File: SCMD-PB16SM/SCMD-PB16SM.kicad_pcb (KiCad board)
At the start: 2 copper layers, 200 x 100 mm, 26 parts, among them M1 SCMD, M10 SCMD, M11 SCMD, M12 SCMD, M2 SCMD, M3 SCMD, M4 SCMD, M5 SCMD, M6 SCMD, M7 SCMD, M8 SCMD, M9 SCMD

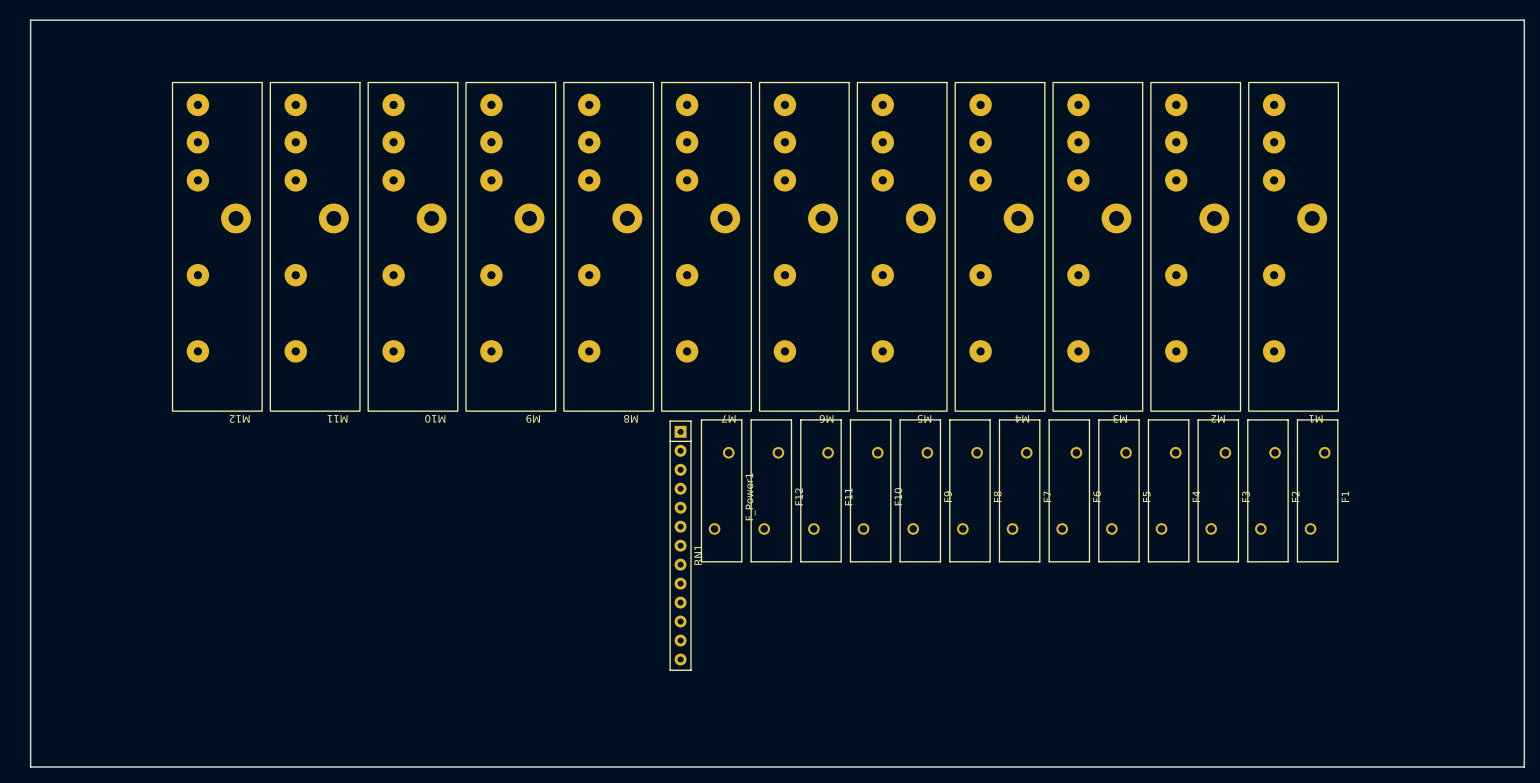
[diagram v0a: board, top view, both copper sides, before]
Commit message: Add files via upload
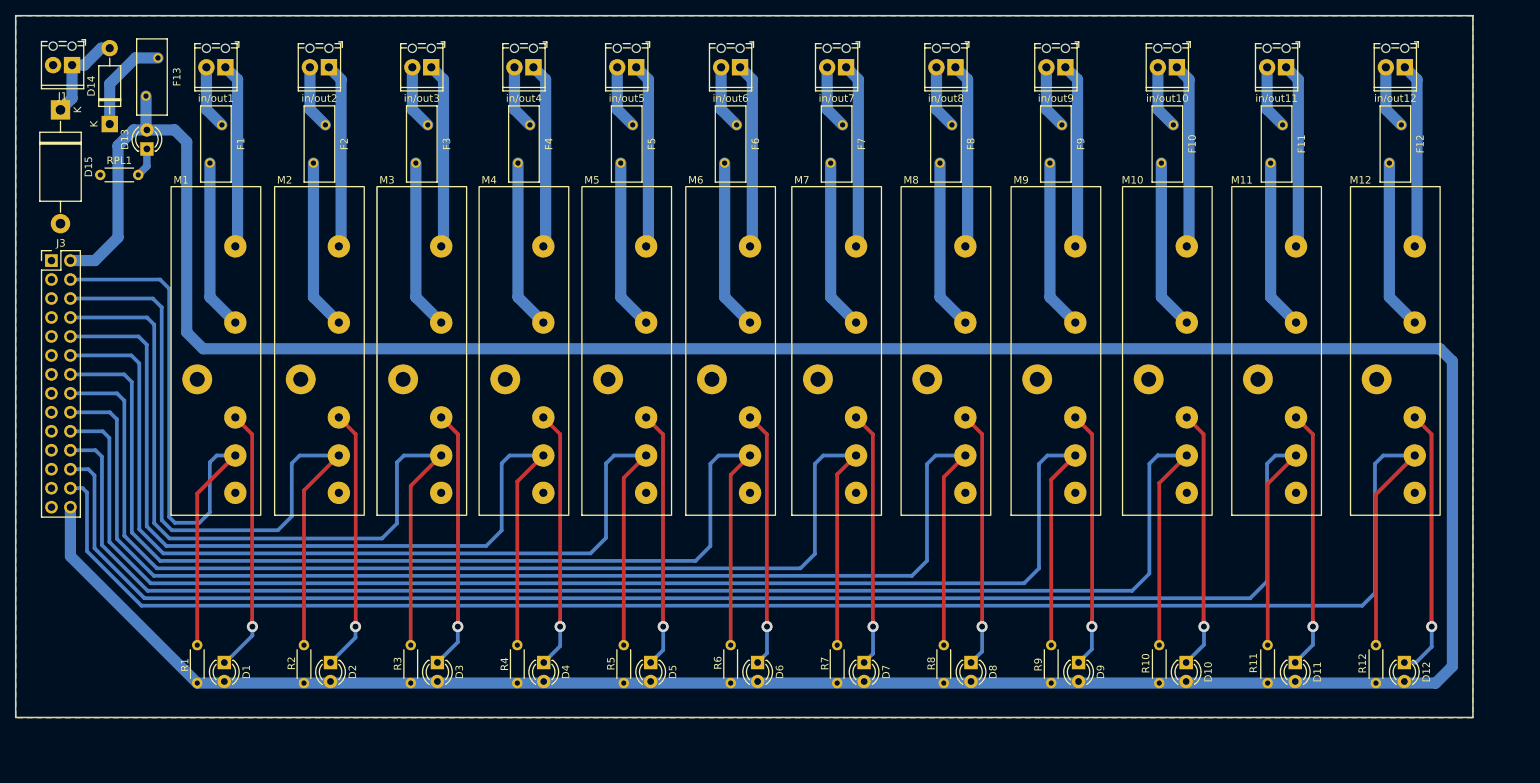
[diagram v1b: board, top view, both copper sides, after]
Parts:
- removed RN1: R_Network12, Resistor_THT:R_Array_SIP13
- added D1: LED, LED_THT:LED_D3.0mm_Clear, F.Cu at (53.9, 103.6)
- added D10: LED, LED_THT:LED_D3.0mm_Clear, F.Cu at (182.7, 103.6)
- added D11: LED, LED_THT:LED_D3.0mm_Clear, F.Cu at (197.3, 103.6)
- added D12: LED, LED_THT:LED_D3.0mm_Clear, F.Cu at (211.9, 103.6)
- added D13: LED, LED_THT:LED_D3.0mm_Clear, F.Cu at (43.6, 34.8)
- added D14: 1N4001, Diode_THT:D_DO-41_SOD81_P10.16mm_Horizontal, F.Cu at (38.6, 31.5)
- added D15: 1N62xxA, Diode_THT:D_DO-201AE_P15.24mm_Horizontal, F.Cu at (32.0, 29.6)
- added D2: LED, LED_THT:LED_D3.0mm_Clear, F.Cu at (68.2, 103.6)
- added D3: LED, LED_THT:LED_D3.0mm_Clear, F.Cu at (82.5, 103.6)
- added D4: LED, LED_THT:LED_D3.0mm_Clear, F.Cu at (96.7, 103.6)
- added D5: LED, LED_THT:LED_D3.0mm_Clear, F.Cu at (111.0, 103.6)
- added D6: LED, LED_THT:LED_D3.0mm_Clear, F.Cu at (125.3, 103.6)
- added D7: LED, LED_THT:LED_D3.0mm_Clear, F.Cu at (139.6, 103.6)
- added D8: LED, LED_THT:LED_D3.0mm_Clear, F.Cu at (153.9, 103.6)
- added D9: LED, LED_THT:LED_D3.0mm_Clear, F.Cu at (168.3, 103.6)
- added J1: Logic Supply, TerminalBlock_Phoenix:TerminalBlock_Phoenix_MPT-0,5-2-2.54_1x02_P2.54mm_Horizontal, F.Cu at (33.5, 23.6)
- added J3: Edge Connector, Connector_PinHeader_2.54mm:PinHeader_2x14_P2.54mm_Vertical, F.Cu at (30.8, 49.8)
- added R1: 3.3R, Resistor_THT:R_Axial_DIN0204_L3.6mm_D1.6mm_P5.08mm_Horizontal, F.Cu at (50.3, 101.3)
- added R10: 3.3R, Resistor_THT:R_Axial_DIN0204_L3.6mm_D1.6mm_P5.08mm_Horizontal, F.Cu at (179.1, 101.3)
- added R11: 3.3R, Resistor_THT:R_Axial_DIN0204_L3.6mm_D1.6mm_P5.08mm_Horizontal, F.Cu at (193.6, 101.3)
- added R12: 3.3R, Resistor_THT:R_Axial_DIN0204_L3.6mm_D1.6mm_P5.08mm_Horizontal, F.Cu at (208.1, 101.3)
- added R2: 3.3R, Resistor_THT:R_Axial_DIN0204_L3.6mm_D1.6mm_P5.08mm_Horizontal, F.Cu at (64.6, 101.3)
- added R3: 3.3R, Resistor_THT:R_Axial_DIN0204_L3.6mm_D1.6mm_P5.08mm_Horizontal, F.Cu at (78.9, 101.3)
- added R4: 3.3R, Resistor_THT:R_Axial_DIN0204_L3.6mm_D1.6mm_P5.08mm_Horizontal, F.Cu at (93.2, 101.3)
- added R5: 3.3R, Resistor_THT:R_Axial_DIN0204_L3.6mm_D1.6mm_P5.08mm_Horizontal, F.Cu at (107.4, 101.3)
- added R6: 3.3R, Resistor_THT:R_Axial_DIN0204_L3.6mm_D1.6mm_P5.08mm_Horizontal, F.Cu at (121.7, 101.3)
- added R7: 3.3R, Resistor_THT:R_Axial_DIN0204_L3.6mm_D1.6mm_P5.08mm_Horizontal, F.Cu at (136.0, 101.3)
- added R8: 3.3R, Resistor_THT:R_Axial_DIN0204_L3.6mm_D1.6mm_P5.08mm_Horizontal, F.Cu at (150.3, 101.3)
- added R9: 3.3R, Resistor_THT:R_Axial_DIN0204_L3.6mm_D1.6mm_P5.08mm_Horizontal, F.Cu at (164.7, 101.3)
- added RPL1: 3.3R, Resistor_THT:R_Axial_DIN0204_L3.6mm_D1.6mm_P5.08mm_Horizontal, F.Cu at (37.3, 38.3)
- added in/out1: Screw_Terminal_01x02, TerminalBlock_Phoenix:TerminalBlock_Phoenix_MPT-0,5-2-2.54_1x02_P2.54mm_Horizontal, F.Cu at (54.1, 23.9)
- added in/out10: Screw_Terminal_01x02, TerminalBlock_Phoenix:TerminalBlock_Phoenix_MPT-0,5-2-2.54_1x02_P2.54mm_Horizontal, F.Cu at (181.5, 23.9)
- added in/out11: Screw_Terminal_01x02, TerminalBlock_Phoenix:TerminalBlock_Phoenix_MPT-0,5-2-2.54_1x02_P2.54mm_Horizontal, F.Cu at (196.1, 23.9)
- added in/out12: Screw_Terminal_01x02, TerminalBlock_Phoenix:TerminalBlock_Phoenix_MPT-0,5-2-2.54_1x02_P2.54mm_Horizontal, F.Cu at (212.0, 23.9)
- added in/out2: Screw_Terminal_01x02, TerminalBlock_Phoenix:TerminalBlock_Phoenix_MPT-0,5-2-2.54_1x02_P2.54mm_Horizontal, F.Cu at (67.9, 23.9)
- added in/out3: Screw_Terminal_01x02, TerminalBlock_Phoenix:TerminalBlock_Phoenix_MPT-0,5-2-2.54_1x02_P2.54mm_Horizontal, F.Cu at (81.6, 23.9)
- added in/out4: Screw_Terminal_01x02, TerminalBlock_Phoenix:TerminalBlock_Phoenix_MPT-0,5-2-2.54_1x02_P2.54mm_Horizontal, F.Cu at (95.3, 23.9)
- added in/out5: Screw_Terminal_01x02, TerminalBlock_Phoenix:TerminalBlock_Phoenix_MPT-0,5-2-2.54_1x02_P2.54mm_Horizontal, F.Cu at (109.1, 23.9)
- added in/out6: Screw_Terminal_01x02, TerminalBlock_Phoenix:TerminalBlock_Phoenix_MPT-0,5-2-2.54_1x02_P2.54mm_Horizontal, F.Cu at (123.0, 23.9)
- added in/out7: Screw_Terminal_01x02, TerminalBlock_Phoenix:TerminalBlock_Phoenix_MPT-0,5-2-2.54_1x02_P2.54mm_Horizontal, F.Cu at (137.2, 23.9)
- added in/out8: Screw_Terminal_01x02, TerminalBlock_Phoenix:TerminalBlock_Phoenix_MPT-0,5-2-2.54_1x02_P2.54mm_Horizontal, F.Cu at (151.8, 23.9)
- added in/out9: Screw_Terminal_01x02, TerminalBlock_Phoenix:TerminalBlock_Phoenix_MPT-0,5-2-2.54_1x02_P2.54mm_Horizontal, F.Cu at (166.6, 23.9)
- F1, F10, F11, F12, F2, F3, F4, F5, F6, F7, F8, F9: footprint Fuse:Fuse_BelFuse_0ZRE0100FF_L18.7mm_W5.1mm -> Fuse:Fuse_BelFuse_0ZRE0016FF_L9.9mm_W3.8mm
- F13: renamed from F_Power1; footprint Fuse:Fuse_BelFuse_0ZRE0100FF_L18.7mm_W5.1mm -> Fuse:Fuse_BelFuse_0ZRE0016FF_L9.9mm_W3.8mm
- moved M12 158.3 mm to (210.7, 61.9), turned to 90 degrees
- moved F1 154.1 mm to (53.6, 31.6)
- moved M1 145.0 mm to (52.8, 61.9), turned to 90 degrees
- moved F2 134.5 mm to (67.5, 31.6)
- moved M11 129.5 mm to (194.8, 61.9), turned to 90 degrees
- moved M2 118.2 mm to (66.7, 61.9), turned to 90 degrees
- moved F3 115.5 mm to (81.2, 31.6)
- moved M10 102.0 mm to (180.2, 61.9), turned to 90 degrees
- moved F4 97.0 mm to (94.9, 31.6)
- moved F12 94.3 mm to (211.5, 31.6)
- moved F13 92.9 mm to (45.0, 22.7)
- moved M3 91.6 mm to (80.4, 61.9), turned to 90 degrees
- moved F5 79.3 mm to (108.6, 31.6)
- moved F11 75.0 mm to (195.6, 31.6)
- moved M9 74.3 mm to (165.3, 61.9), turned to 90 degrees
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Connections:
- F1 pad 1: unconnected-(F1-Pad1) -> Net-(in/out1-Pin_2)
- F1 pad 2: unconnected-(F1-Pad2) -> Net-(M1--_in_out)
- F10 pad 1: unconnected-(F10-Pad1) -> Net-(in/out10-Pin_2)
- F10 pad 2: unconnected-(F10-Pad2) -> Net-(M10--_in_out)
- F11 pad 1: unconnected-(F11-Pad1) -> Net-(in/out11-Pin_2)
- F11 pad 2: unconnected-(F11-Pad2) -> Net-(M11--_in_out)
- F12 pad 1: unconnected-(F12-Pad1) -> Net-(in/out12-Pin_2)
- F12 pad 2: unconnected-(F12-Pad2) -> Net-(M12--_in_out)
- F13 pad 1: unconnected-(F_Power1-Pad1) -> Net-(D14-K)
- F13 pad 2: unconnected-(F_Power1-Pad2) -> VCC
- F2 pad 1: unconnected-(F2-Pad1) -> Net-(in/out2-Pin_2)
- F2 pad 2: unconnected-(F2-Pad2) -> Net-(M2--_in_out)
- F3 pad 1: unconnected-(F3-Pad1) -> Net-(in/out3-Pin_2)
- F3 pad 2: unconnected-(F3-Pad2) -> Net-(M3--_in_out)
- F4 pad 1: unconnected-(F4-Pad1) -> Net-(in/out4-Pin_2)
- F4 pad 2: unconnected-(F4-Pad2) -> Net-(M4--_in_out)
- F5 pad 1: unconnected-(F5-Pad1) -> Net-(in/out5-Pin_2)
- F5 pad 2: unconnected-(F5-Pad2) -> Net-(M5--_in_out)
- F6 pad 1: unconnected-(F6-Pad1) -> Net-(in/out6-Pin_2)
- F6 pad 2: unconnected-(F6-Pad2) -> Net-(M6--_in_out)
- F7 pad 1: unconnected-(F7-Pad1) -> Net-(in/out7-Pin_2)
- F7 pad 2: unconnected-(F7-Pad2) -> Net-(M7--_in_out)
- F8 pad 1: unconnected-(F8-Pad1) -> Net-(in/out8-Pin_2)
- F8 pad 2: unconnected-(F8-Pad2) -> Net-(M8--_in_out)
- F9 pad 1: unconnected-(F9-Pad1) -> Net-(in/out9-Pin_2)
- F9 pad 2: unconnected-(F9-Pad2) -> Net-(M9--_in_out)
- M1 pad 1: unconnected-(M1-+_in_out-Pad1) -> Net-(M1-+_in_out)
- M1 pad 2: unconnected-(M1--_in_out-Pad2) -> Net-(M1--_in_out)
- M1 pad 3: unconnected-(M1-+_5v_dc_logic-Pad3) -> Net-(D1-K)
- M1 pad 4: unconnected-(M1-+_logic_in_out-Pad4) -> /J3-4
- M1 pad 5: unconnected-(M1--_logic_in_out-Pad5) -> GND
- M10 pad 1: unconnected-(M10-+_in_out-Pad1) -> Net-(M10-+_in_out)
- M10 pad 2: unconnected-(M10--_in_out-Pad2) -> Net-(M10--_in_out)
- M10 pad 3: unconnected-(M10-+_5v_dc_logic-Pad3) -> Net-(D10-K)
- M10 pad 4: unconnected-(M10-+_logic_in_out-Pad4) -> /J3-22
- M10 pad 5: unconnected-(M10--_logic_in_out-Pad5) -> GND
- M11 pad 1: unconnected-(M11-+_in_out-Pad1) -> Net-(M11-+_in_out)
- M11 pad 2: unconnected-(M11--_in_out-Pad2) -> Net-(M11--_in_out)
- M11 pad 3: unconnected-(M11-+_5v_dc_logic-Pad3) -> Net-(D11-K)
- M11 pad 4: unconnected-(M11-+_logic_in_out-Pad4) -> /J3-24
- M11 pad 5: unconnected-(M11--_logic_in_out-Pad5) -> GND
- M12 pad 1: unconnected-(M12-+_in_out-Pad1) -> Net-(M12-+_in_out)
- M12 pad 2: unconnected-(M12--_in_out-Pad2) -> Net-(M12--_in_out)
- M12 pad 3: unconnected-(M12-+_5v_dc_logic-Pad3) -> Net-(D12-K)
- M12 pad 4: unconnected-(M12-+_logic_in_out-Pad4) -> /J3-26
- M12 pad 5: unconnected-(M12--_logic_in_out-Pad5) -> GND
- M2 pad 1: unconnected-(M2-+_in_out-Pad1) -> Net-(M2-+_in_out)
- M2 pad 2: unconnected-(M2--_in_out-Pad2) -> Net-(M2--_in_out)
- M2 pad 3: unconnected-(M2-+_5v_dc_logic-Pad3) -> Net-(D2-K)
- M2 pad 4: unconnected-(M2-+_logic_in_out-Pad4) -> /J3-6
- M2 pad 5: unconnected-(M2--_logic_in_out-Pad5) -> GND
- M3 pad 1: unconnected-(M3-+_in_out-Pad1) -> Net-(M3-+_in_out)
- M3 pad 2: unconnected-(M3--_in_out-Pad2) -> Net-(M3--_in_out)
- M3 pad 3: unconnected-(M3-+_5v_dc_logic-Pad3) -> Net-(D3-K)
- M3 pad 4: unconnected-(M3-+_logic_in_out-Pad4) -> /J3-8
- M3 pad 5: unconnected-(M3--_logic_in_out-Pad5) -> GND
- M4 pad 1: unconnected-(M4-+_in_out-Pad1) -> Net-(M4-+_in_out)
- M4 pad 2: unconnected-(M4--_in_out-Pad2) -> Net-(M4--_in_out)
- M4 pad 3: unconnected-(M4-+_5v_dc_logic-Pad3) -> Net-(D4-K)
- M4 pad 4: unconnected-(M4-+_logic_in_out-Pad4) -> /J3-10
- M4 pad 5: unconnected-(M4--_logic_in_out-Pad5) -> GND
- M5 pad 1: unconnected-(M5-+_in_out-Pad1) -> Net-(M5-+_in_out)
- M5 pad 2: unconnected-(M5--_in_out-Pad2) -> Net-(M5--_in_out)
- M5 pad 3: unconnected-(M5-+_5v_dc_logic-Pad3) -> Net-(D5-K)
- M5 pad 4: unconnected-(M5-+_logic_in_out-Pad4) -> /J3-12
- M5 pad 5: unconnected-(M5--_logic_in_out-Pad5) -> GND
- M6 pad 1: unconnected-(M6-+_in_out-Pad1) -> Net-(M6-+_in_out)
- M6 pad 2: unconnected-(M6--_in_out-Pad2) -> Net-(M6--_in_out)
- M6 pad 3: unconnected-(M6-+_5v_dc_logic-Pad3) -> Net-(D6-K)
- M6 pad 4: unconnected-(M6-+_logic_in_out-Pad4) -> /J3-14
- M6 pad 5: unconnected-(M6--_logic_in_out-Pad5) -> GND
- M7 pad 1: unconnected-(M7-+_in_out-Pad1) -> Net-(M7-+_in_out)
- M7 pad 2: unconnected-(M7--_in_out-Pad2) -> Net-(M7--_in_out)
- M7 pad 3: unconnected-(M7-+_5v_dc_logic-Pad3) -> Net-(D7-K)
- M7 pad 4: unconnected-(M7-+_logic_in_out-Pad4) -> /J3-16
- M7 pad 5: unconnected-(M7--_logic_in_out-Pad5) -> GND
- M8 pad 1: unconnected-(M8-+_in_out-Pad1) -> Net-(M8-+_in_out)
- M8 pad 2: unconnected-(M8--_in_out-Pad2) -> Net-(M8--_in_out)
- M8 pad 3: unconnected-(M8-+_5v_dc_logic-Pad3) -> Net-(D8-K)
- M8 pad 4: unconnected-(M8-+_logic_in_out-Pad4) -> /J3-18
- M8 pad 5: unconnected-(M8--_logic_in_out-Pad5) -> GND
- M9 pad 1: unconnected-(M9-+_in_out-Pad1) -> Net-(M9-+_in_out)
- M9 pad 2: unconnected-(M9--_in_out-Pad2) -> Net-(M9--_in_out)
- M9 pad 3: unconnected-(M9-+_5v_dc_logic-Pad3) -> Net-(D9-K)
- M9 pad 4: unconnected-(M9-+_logic_in_out-Pad4) -> /J3-20
- M9 pad 5: unconnected-(M9--_logic_in_out-Pad5) -> GND
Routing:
- net VCC: track 0.00 -> 472.3 mm
- net /J3-26: track 0.00 -> 237.1 mm
- net /J3-24: track 0.00 -> 221.1 mm
- net /J3-22: track 0.00 -> 207.2 mm
- net /J3-20: track 0.00 -> 193.1 mm
- net /J3-18: track 0.00 -> 179.1 mm
- net /J3-16: track 0.00 -> 165.3 mm
- net /J3-14: track 0.00 -> 151.9 mm
- net /J3-12: track 0.00 -> 139.0 mm
- net /J3-10: track 0.00 -> 126.3 mm
- net /J3-8: track 0.00 -> 113.9 mm
- net /J3-6: track 0.00 -> 101.1 mm
- net /J3-4: track 0.00 -> 88.7 mm
- net Net-(D12-K): track 0.00 -> 35.4 mm, vias 0 -> 1
- net Net-(D1-K): track 0.00 -> 34.6 mm, vias 0 -> 1
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- added copper zone on B.Cu, net GND
- added copper zone on F.Cu, net GND
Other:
- board size 200 x 100 mm -> 195.1 x 94 mm
